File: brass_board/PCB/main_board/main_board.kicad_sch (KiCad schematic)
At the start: 142 parts

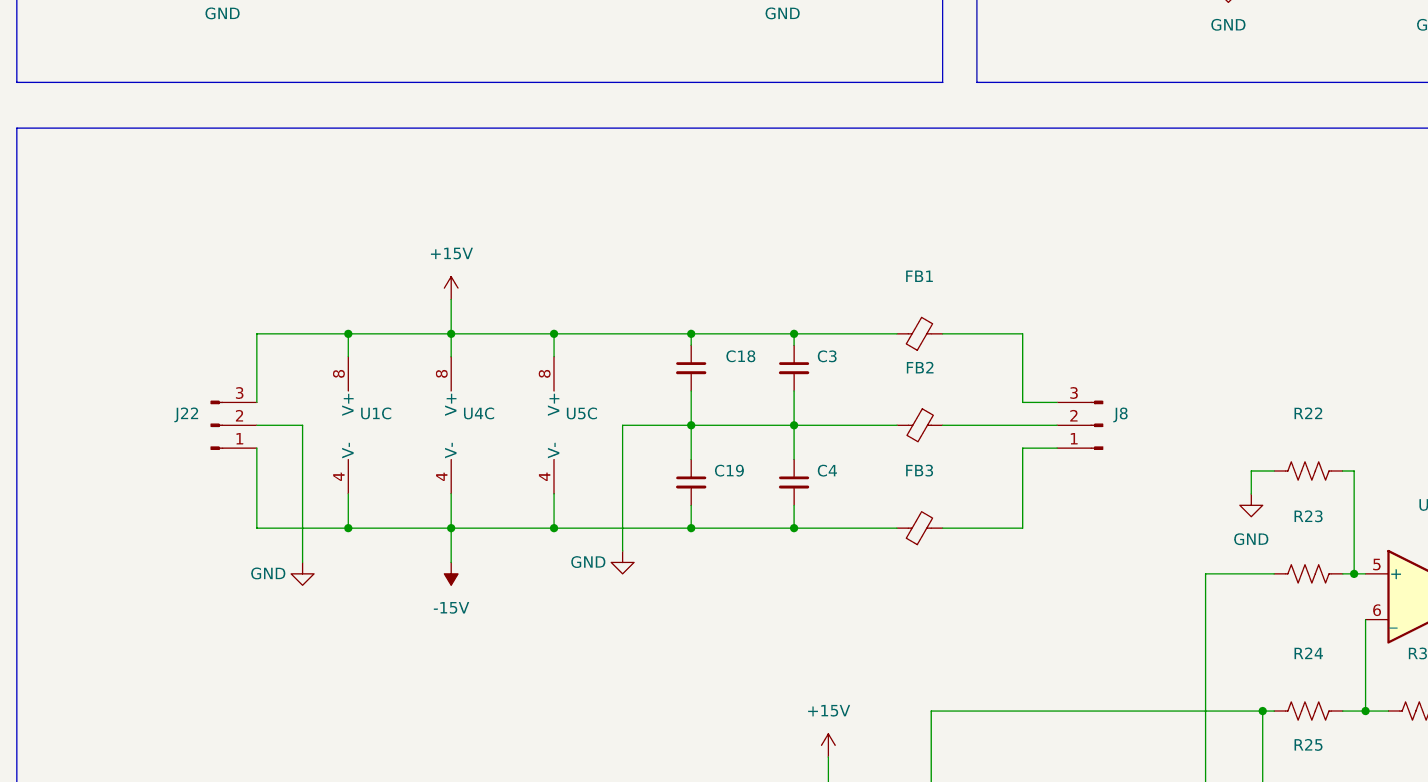
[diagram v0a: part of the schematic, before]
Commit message: Sent to Fab
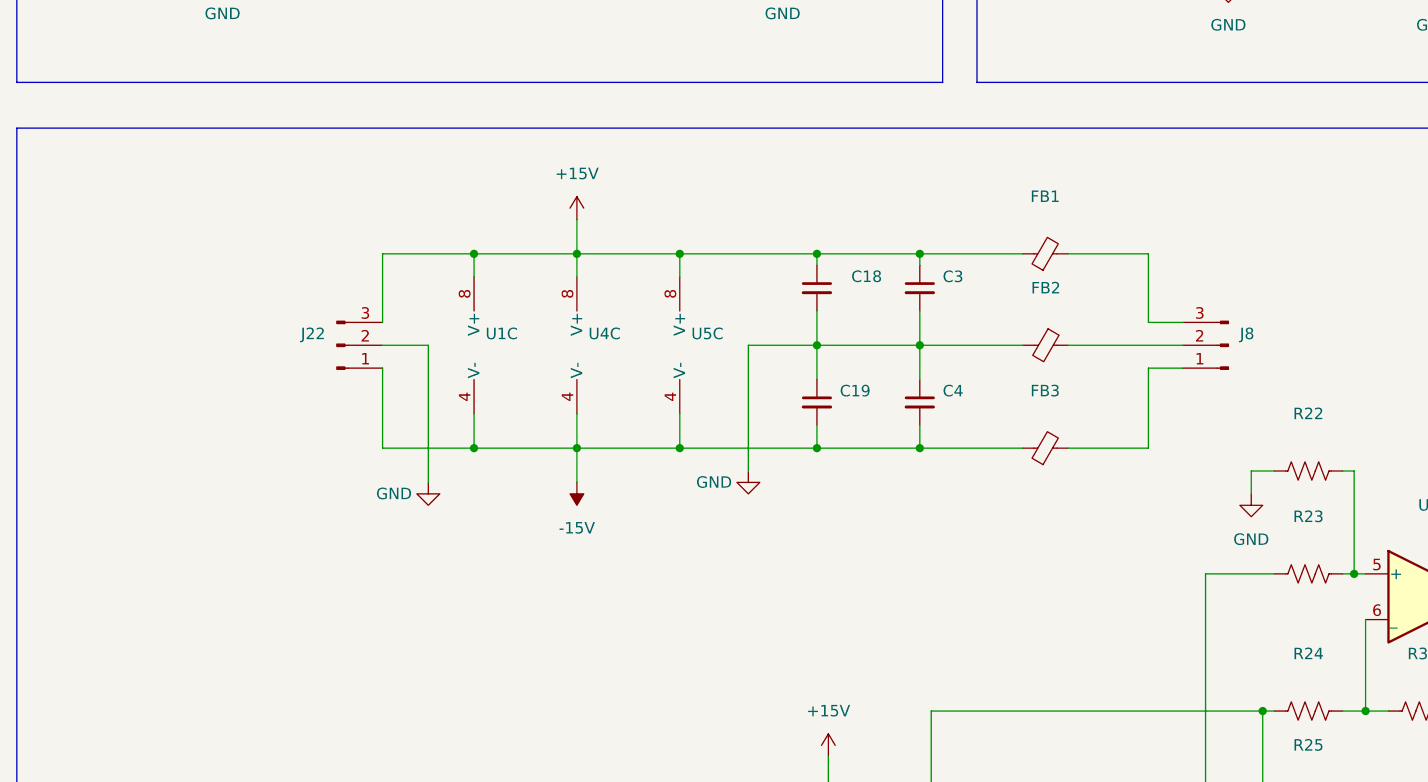
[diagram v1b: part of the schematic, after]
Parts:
- J11: LCSC C124378 -> (none)
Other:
- moved on the sheet: C18, C19, C3, C4, FB1, FB2, FB3, J22, J8, U1C, U4C, U5C
